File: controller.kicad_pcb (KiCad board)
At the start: 2 copper layers, 81 x 35 mm, 28 parts, among them SW1 SW_Push, U1 PRTR5V0U2X, U2 AT90USB1286-AU, Y1 16MHz

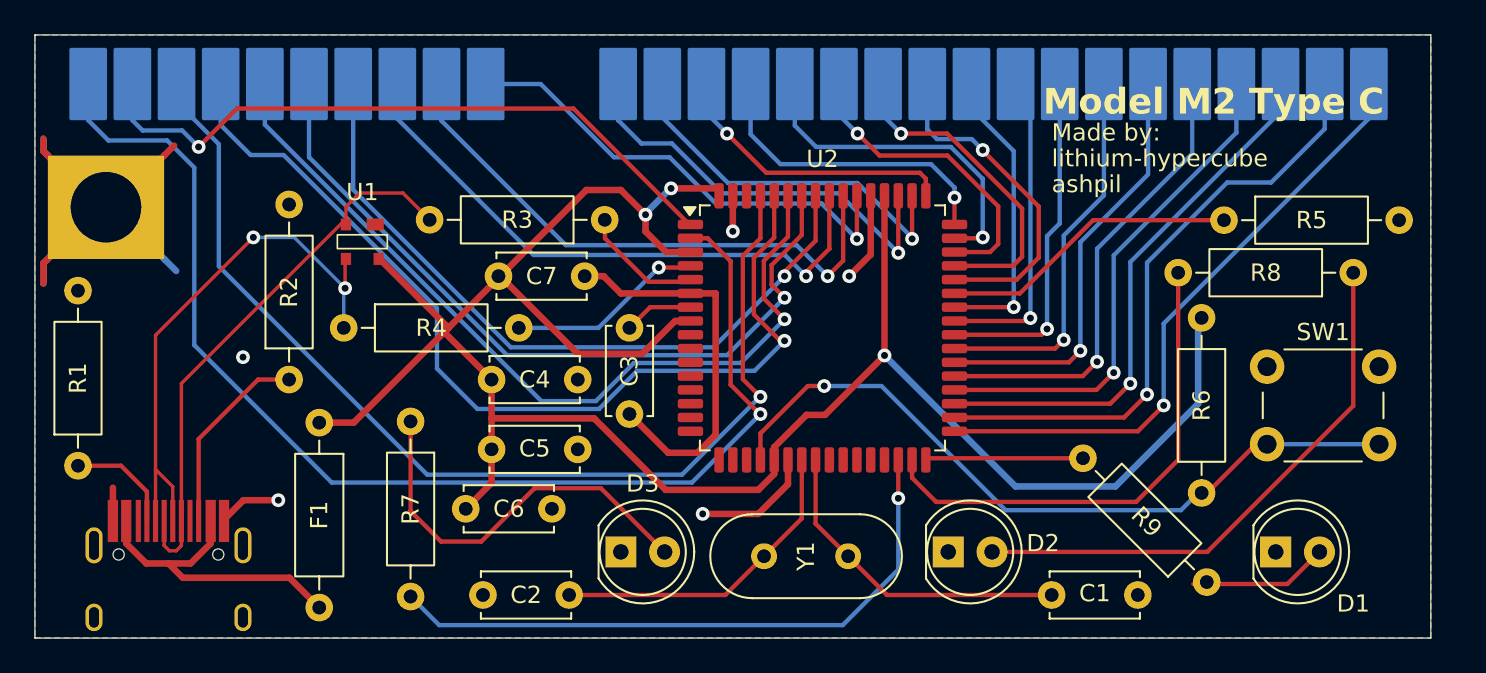
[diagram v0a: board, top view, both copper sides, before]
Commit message: Add a trace
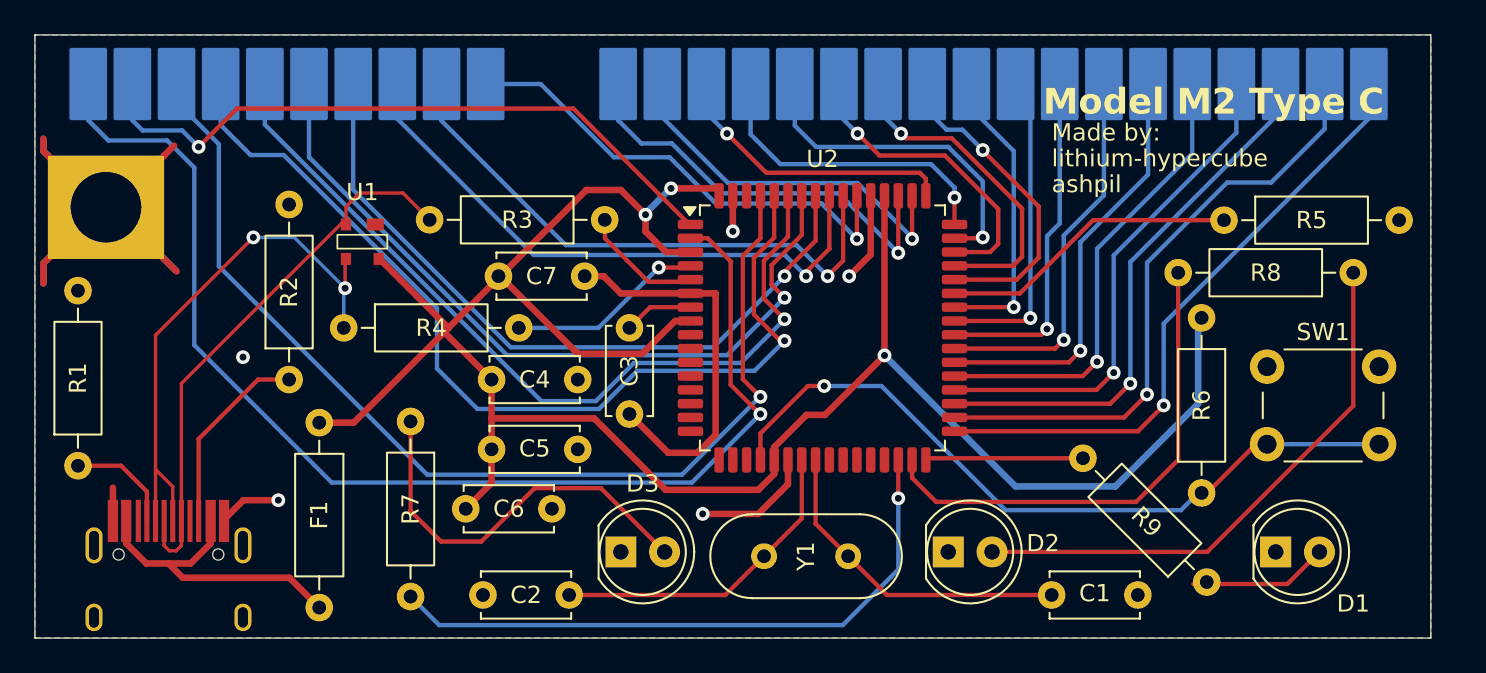
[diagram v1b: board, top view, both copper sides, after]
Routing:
- net GND: track 76.1 -> 81.0 mm
- net 1: track 19.3 -> 18.7 mm
